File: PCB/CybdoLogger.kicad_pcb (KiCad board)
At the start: 2 copper layers, 16 x 50 mm, 33 parts, among them SW2 READ, U1 RP2040, U2 USBLC6-2SC6, U3 USBLC6-2SC6, U4 MCP1700x-330xxTT, U5 W25Q16JVUXIQ, Y1 Crystal_GND24

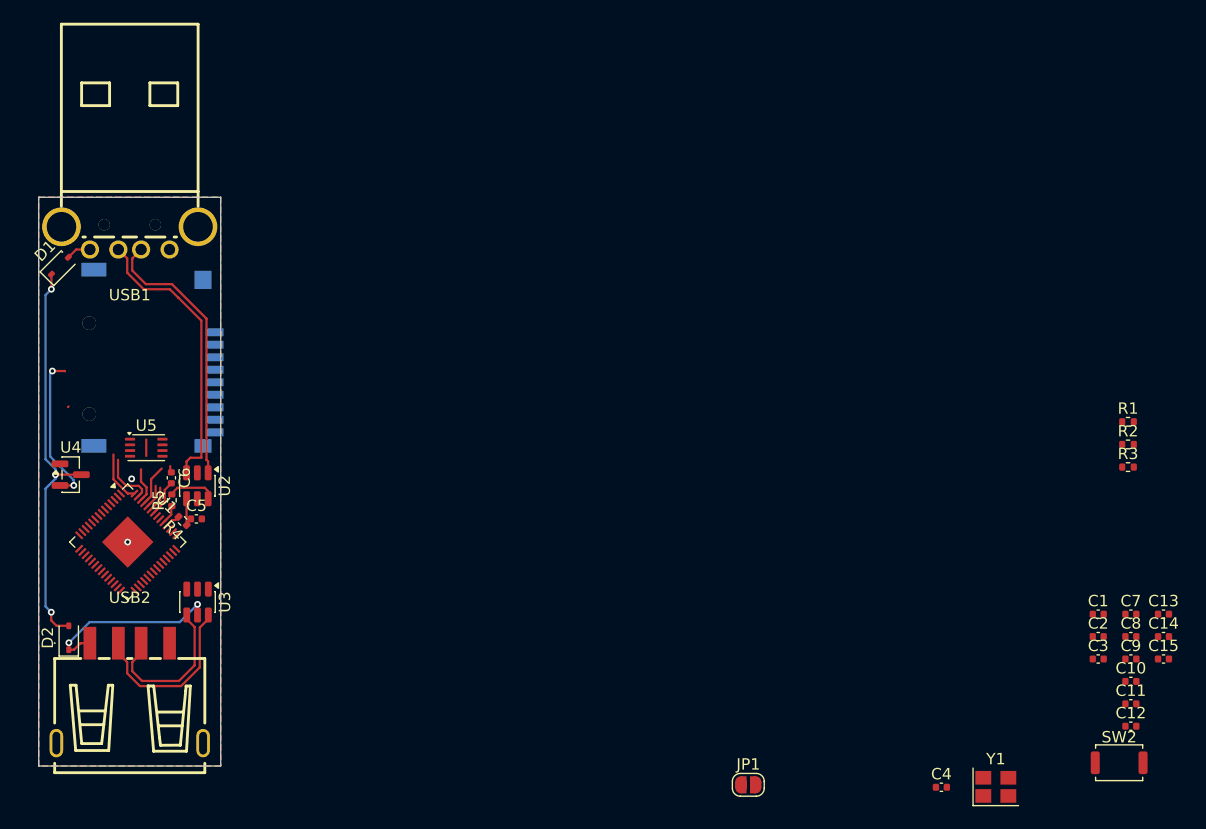
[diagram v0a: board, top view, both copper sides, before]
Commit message: mroe rounting
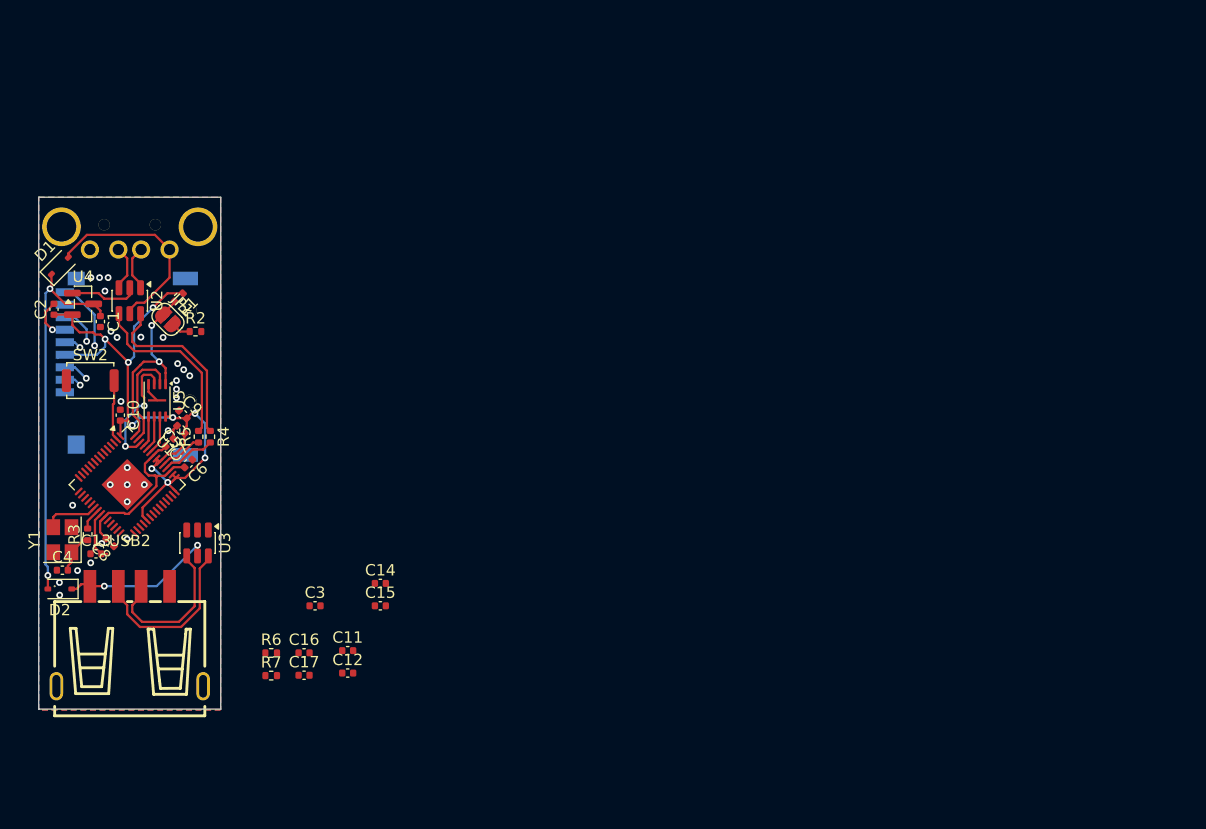
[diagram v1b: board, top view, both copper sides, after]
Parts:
- added C16: 100nF, Capacitor_SMD:C_0402_1005Metric, F.Cu at (65.3, 86.0)
- added C17: 10uF, Capacitor_SMD:C_0402_1005Metric, F.Cu at (65.3, 87.9)
- added R6: 10kR, Resistor_SMD:R_0402_1005Metric, F.Cu at (62.4, 86.0)
- added R7: 10kR, Resistor_SMD:R_0402_1005Metric, F.Cu at (62.4, 88.0)
- USB1: moved to B.Cu
- moved SW2 96.5 mm to (46.5, 62.0)
- moved C2 96.2 mm to (43.3, 55.8), turned to 90 degrees
- moved C13 94.0 mm to (47.0, 77.2)
- moved C10 91.9 mm to (49.2, 65.1), turned to -90 degrees
- moved R3 91.6 mm to (46.3, 75.5), turned to 90 degrees
- moved C1 91.4 mm to (47.4, 56.8), turned to -90 degrees
- moved C8 90.1 mm to (48.3, 76.2), turned to 135 degrees
- moved C9 86.1 mm to (54.7, 65.0), turned to -45 degrees
- moved C7 85.8 mm to (53.5, 67.5), turned to -135 degrees
- moved Y1 84.9 mm to (44.1, 76.0), turned to 90 degrees
- moved R1 84.2 mm to (54.3, 54.7), turned to -135 degrees
- moved R2 82.6 mm to (55.8, 57.7)
- moved C4 79.6 mm to (44.1, 78.7)
- moved C11 69.0 mm to (69.2, 85.8)
- moved C12 69.0 mm to (69.2, 87.7)
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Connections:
- U1 pad 2: unconnected-(U1-GPIO0-Pad2) -> /READ_SD
- U2 pad 1: /UD+ -> /UD-
- U2 pad 3: /UD- -> /UD+
- U2 pad 4: /USB_UP_D- -> /USB_UP_D+
- U2 pad 6: /USB_UP_D+ -> /USB_UP_D-
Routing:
- net +3V3: track 13.3 -> 64.9 mm, vias 2 -> 9
- net /UD-: track 25.2 -> 3.98 mm
- net /UD+: track 24.3 -> 4.09 mm
- net VBUS: track 2.21 -> 17.9 mm
- net +1V1: track 3.23 -> 16.7 mm, vias 0 -> 1
- net /USB_UP_D-: track 2.32 -> 15.8 mm
- net /BOOTSEL: track 4.55 -> 17.3 mm, vias 0 -> 2
- net GND: track 0.44 -> 11.9 mm, vias 2 -> 28
- net /USB_UP_D+: track 4.38 -> 15.8 mm
- net /FLASH_SD2: track 3.11 -> 10.4 mm, vias 0 -> 2
- net /SD_CD: track 0.00 -> 6.17 mm, vias 0 -> 1
- net /READ_SD: track 0.00 -> 5.37 mm
- net Net-(U1-XIN): track 0.00 -> 4.89 mm
- net /FLASH_SD1: track 4.91 -> 9.35 mm
- net Net-(C4-Pad2): track 0.00 -> 3.57 mm
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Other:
- board size 16 x 50 mm -> 16 x 45 mm
